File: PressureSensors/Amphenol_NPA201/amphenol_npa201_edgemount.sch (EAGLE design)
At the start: 5 parts

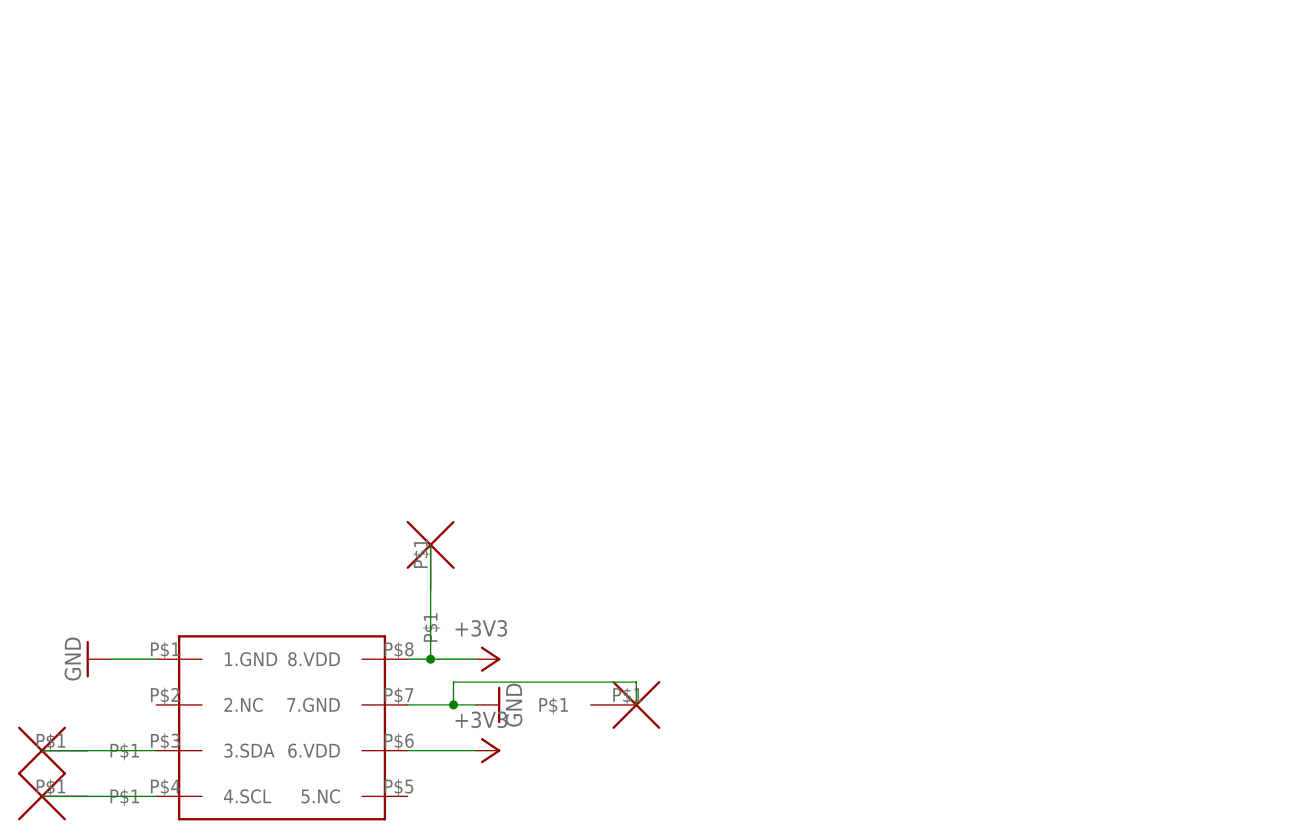
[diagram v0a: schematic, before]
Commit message: overdue commit
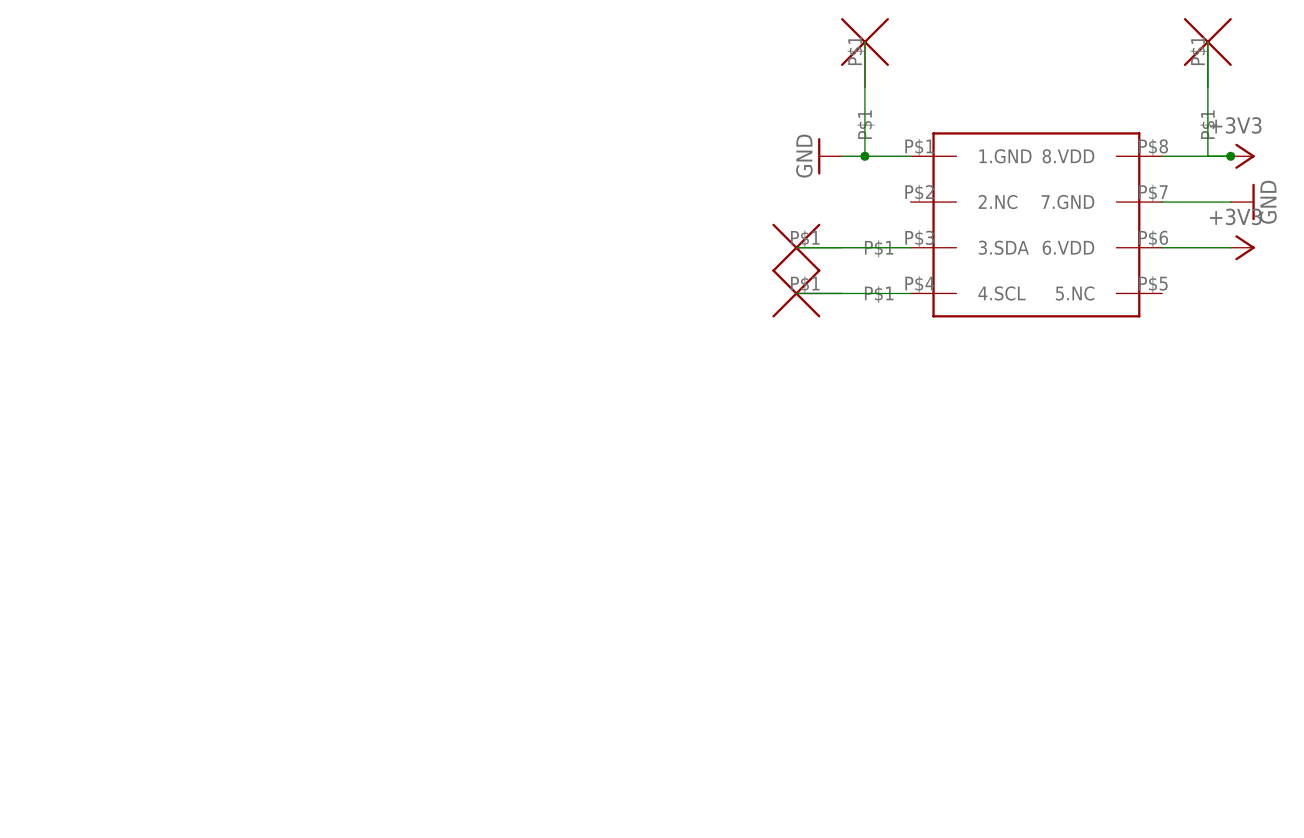
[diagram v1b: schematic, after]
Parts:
- U$1: value AMPHENOL_NPA201 -> AMPHENOL_NPA201EDGEMOUNT; device Amphenol_NPA201:AMPHENOL_NPA201 -> Sombeck_lib:AMPHENOL_NPA201EDGEMOUNT
- U$2, U$3, U$4, U$5: value WIREPAD_0,8/0,45 -> WIREPADWIREPAD_0,5/0,3; device wirepad_08-045:WIREPAD_0,8/0,45 -> Sombeck_lib:WIREPADWIREPAD_0,5/0,3
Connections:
- net +3V3: now also U$5.P$1; no longer U$4.P$1
- net GND: now also U$4.P$1; no longer U$5.P$1
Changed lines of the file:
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@@
 <layers>
 <layer number="1" name="Top" color="4" fill="1" visible="no" active="no"/>
-<layer number="2" name="Route2" color="1" fill="3" visible="no" active="no"/>
-<layer number="3" name="Route3" color="4" fill="3" visible="no" active="no"/>
-<layer number="4" name="Route4" color="1" fill="4" visible="no" active="no"/>
-<layer number="5" name="Route5" color="4" fill="4" visible="no" active="no"/>
-<layer number="6" name="Route6" color="1" fill="8" visible="no" active="no"/>
-<layer number="7" name="Route7" color="4" fill="8" visible="no" active="no"/>
-<layer number="8" name="Route8" color="1" fill="2" visible="no" active="no"/>
-<layer number="9" name="Route9" color="4" fill="2" visible="no" active="no"/>
-<layer number="10" name="Route10" color="1" fill="7" visible="no" active="no"/>
-<layer number="11" name="Route11" color="4" fill="7" visible="no" active="no"/>
-<layer number="12" name="Route12" color="1" fill="5" visible="no" active="no"/>
-<layer number="13" name="Route13" color="4" fill="5" visible="no" active="no"/>
-<layer number="14" name="Route14" color="1" fill="6" visible="no" active="no"/>
-<layer number="15" name="Route15" color="4" fill="6" visible="no" active="no"/>
 <layer number="16" name="Bottom" color="1" fill="1" visible="no" active="no"/>
 <layer number="17" name="Pads" color="2" fill="1" visible="no" active="no"/>
@@
 </classes>
 <parts>
-<part name="U$1" library="Amphenol_NPA201" deviceset="AMPHENOL_NPA201" device=""/>
 <part name="+3V1" library="supply1" library_urn="urn:adsk.eagle:library:371" deviceset="+3V3" device=""/>
 <part name="+3V2" library="supply1" library_urn="urn:adsk.eagle:library:371" deviceset="+3V3" device=""/>
 <part name="GND1" library="supply1" library_urn="urn:adsk.eagle:library:371" deviceset="GND" device=""/>
 <part name="GND2" library="supply1" library_urn="urn:adsk.eagle:library:371" deviceset="GND" device=""/>
-<part name="U$2" library="wirepad_08-045" deviceset="WIREPAD_0,8/0,45" device=""/>
-<part name="U$3" library="wirepad_08-045" deviceset="WIREPAD_0,8/0,45" device=""/>
-<part name="U$4" library="wirepad_08-045" deviceset="WIREPAD_0,8/0,45" device=""/>
-<part name="U$5" library="wirepad_08-045" deviceset="WIREPAD_0,8/0,45" device=""/>
+<part name="U$2" library="Sombeck_lib" deviceset="WIREPAD" device="WIREPAD_0,5/0,3"/>
+<part name="U$3" library="Sombeck_lib" deviceset="WIREPAD" device="WIREPAD_0,5/0,3"/>
+<part name="U$4" library="Sombeck_lib" deviceset="WIREPAD" device="WIREPAD_0,5/0,3"/>
+<part name="U$5" library="Sombeck_lib" deviceset="WIREPAD" device="WIREPAD_0,5/0,3"/>
+<part name="U$1" library="Sombeck_lib" deviceset="AMPHENOL_NPA201" device="EDGEMOUNT"/>
 </parts>
 <sheets>
@@
 </plain>
 <instances>
-<instance part="U$1" gate="G$1" x="0" y="2.54"/>
-<instance part="+3V1" gate="G$1" x="25.4" y="7.62" rot="R270"/>
-<instance part="+3V2" gate="G$1" x="25.4" y="-2.54" rot="R270"/>
-<instance part="GND1" gate="1" x="25.4" y="2.54" rot="R90"/>
-<instance part="GND2" gate="1" x="-20.32" y="7.62" rot="R270"/>
-<instance part="U$2" gate="G$1" x="-20.32" y="-2.54"/>
-<instance part="U$3" gate="G$1" x="-20.32" y="-7.62"/>
-<instance part="U$4" gate="G$1" x="17.78" y="15.24" rot="R270"/>
-<instance part="U$5" gate="G$1" x="35.56" y="2.54" rot="R180"/>
+<instance part="+3V1" gate="G$1" x="109.22" y="63.5" rot="R270"/>
+<instance part="+3V2" gate="G$1" x="109.22" y="53.34" rot="R270"/>
+<instance part="GND1" gate="1" x="60.96" y="63.5" rot="R270"/>
+<instance part="GND2" gate="1" x="109.22" y="58.42" rot="R90"/>
+<instance part="U$2" gate="G$1" x="63.5" y="53.34"/>
+<instance part="U$3" gate="G$1" x="63.5" y="48.26"/>
+<instance part="U$4" gate="G$1" x="66.04" y="71.12" rot="R270"/>
+<instance part="U$5" gate="G$1" x="104.14" y="71.12" rot="R270"/>
+<instance part="U$1" gate="G$1" x="83.82" y="58.42"/>
 </instances>
 <busses>
@@
 <net name="GND" class="0">
 <segment>
-<pinref part="GND2" gate="1" pin="GND"/>
+<pinref part="GND1" gate="1" pin="GND"/>
+<wire x1="63.5" y1="63.5" x2="66.04" y2="63.5" width="0.1524" layer="91"/>
+<pinref part="U$4" gate="G$1" pin="P$1"/>
+<wire x1="66.04" y1="63.5" x2="71.12" y2="63.5" width="0.1524" layer="91"/>
+<wire x1="66.04" y1="63.5" x2="66.04" y2="76.2" width="0.1524" layer="91"/>
+<junction x="66.04" y="63.5"/>
 <pinref part="U$1" gate="G$1" pin="1.GND"/>
-<wire x1="-17.78" y1="7.62" x2="-12.7" y2="7.62" width="0.1524" layer="91"/>
 </segment>
 <segment>
+<pinref part="GND2" gate="1" pin="GND"/>
+<wire x1="99.06" y1="58.42" x2="106.68" y2="58.42" width="0.1524" layer="91"/>
 <pinref part="U$1" gate="G$1" pin="7.GND"/>
-<pinref part="GND1" gate="1" pin="GND"/>
-<wire x1="15.24" y1="2.54" x2="20.32" y2="2.54" width="0.1524" layer="91"/>
-<wire x1="20.32" y1="2.54" x2="22.86" y2="2.54" width="0.1524" layer="91"/>
-<wire x1="20.32" y1="2.54" x2="20.32" y2="5.08" width="0.1524" layer="91"/>
-<junction x="20.32" y="2.54"/>
-<wire x1="20.32" y1="5.08" x2="40.64" y2="5.08" width="0.1524" layer="91"/>
+</segment>
+</net>
+<net name="+3V3" class="0">
+<segment>
+<pinref part="+3V1" gate="G$1" pin="+3V3"/>
+<wire x1="99.06" y1="63.5" x2="106.68" y2="63.5" width="0.1524" layer="91"/>
 <pinref part="U$5" gate="G$1" pin="P$1"/>
-<wire x1="40.64" y1="5.08" x2="40.64" y2="2.54" width="0.1524" layer="91"/>
+<wire x1="106.68" y1="63.5" x2="104.14" y2="63.5" width="0.1524" layer="91"/>
+<wire x1="104.14" y1="63.5" x2="104.14" y2="76.2" width="0.1524" layer="91"/>
+<junction x="106.68" y="63.5"/>
+<pinref part="U$1" gate="G$1" pin="8.VDD"/>
+</segment>
+<segment>
+<pinref part="+3V2" gate="G$1" pin="+3V3"/>
+<wire x1="99.06" y1="53.34" x2="106.68" y2="53.34" width="0.1524" layer="91"/>
+<pinref part="U$1" gate="G$1" pin="6.VDD"/>
 </segment>
 </net>
 <net name="N$1" class="0">
 <segment>
+<pinref part="U$2" gate="G$1" pin="P$1"/>
+<wire x1="58.42" y1="53.34" x2="71.12" y2="53.34" width="0.1524" layer="91"/>
 <pinref part="U$1" gate="G$1" pin="3.SDA"/>
-<pinref part="U$2" gate="G$1" pin="P$1"/>
-<wire x1="-12.7" y1="-2.54" x2="-25.4" y2="-2.54" width="0.1524" layer="91"/>
 </segment>
 </net>
@@
 <segment>
 <pinref part="U$3" gate="G$1" pin="P$1"/>
+<wire x1="58.42" y1="48.26" x2="71.12" y2="48.26" width="0.1524" layer="91"/>
 <pinref part="U$1" gate="G$1" pin="4.SCL"/>
-<wire x1="-25.4" y1="-7.62" x2="-12.7" y2="-7.62" width="0.1524" layer="91"/>
 </segment>
 </net>
-<net name="+3V3" class="0">
-<segment>
-<pinref part="U$1" gate="G$1" pin="6.VDD"/>
-<pinref part="+3V2" gate="G$1" pin="+3V3"/>
-<wire x1="15.24" y1="-2.54" x2="22.86" y2="-2.54" width="0.1524" layer="91"/>
-</segment>
-<segment>
-<pinref part="U$1" gate="G$1" pin="8.VDD"/>
-<pinref part="+3V1" gate="G$1" pin="+3V3"/>
-<wire x1="15.24" y1="7.62" x2="17.78" y2="7.62" width="0.1524" layer="91"/>
-<pinref part="U$4" gate="G$1" pin="P$1"/>
-<wire x1="17.78" y1="7.62" x2="22.86" y2="7.62" width="0.1524" layer="91"/>
-<wire x1="17.78" y1="20.32" x2="17.78" y2="7.62" width="0.1524" layer="91"/>
-<junction x="17.78" y="7.62"/>
-</segment>
-</net>
